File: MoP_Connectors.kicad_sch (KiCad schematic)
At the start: 1 part, among them J22 Conn_02x22_Top_Bottom

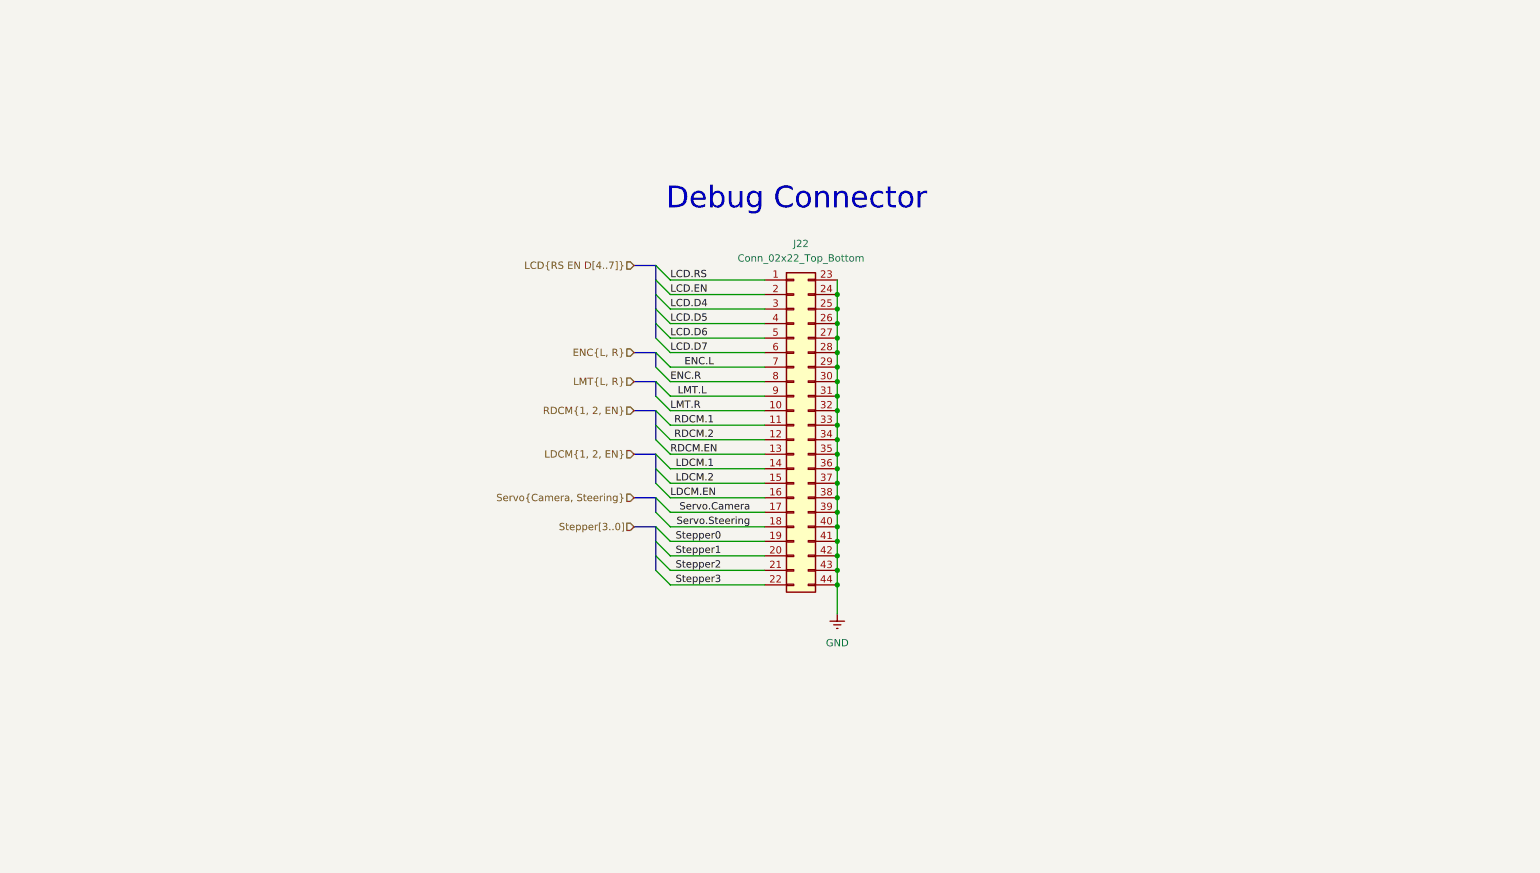
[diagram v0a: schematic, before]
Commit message: Finished schematics
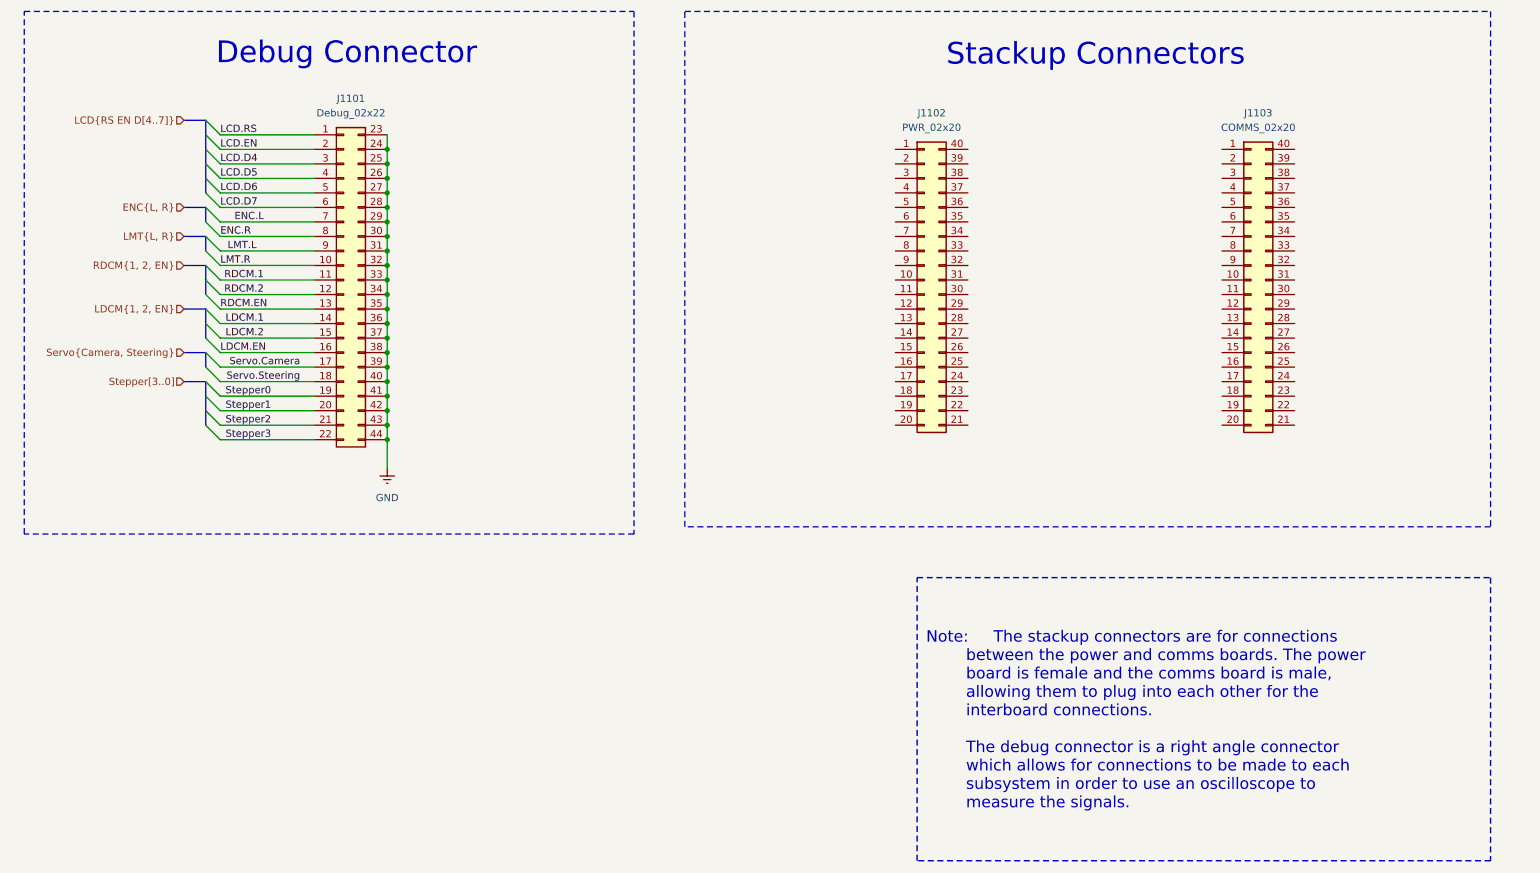
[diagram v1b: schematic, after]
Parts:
- added J1102: PWR_02x20, Connector_PinHeader_2.54mm:PinHeader_2x20_P2.54mm_Vertical, symbol Connector_Generic:Conn_02x20_Counter_Clockwise
- added J1103: COMMS_02x20, Connector_PinHeader_2.54mm:PinHeader_2x20_P2.54mm_Vertical, symbol Connector_Generic:Conn_02x20_Counter_Clockwise
- J1101: renamed from J22; value Conn_02x22_Top_Bottom -> Debug_02x22; footprint (none) -> Connector_PinHeader_1.00mm:PinHeader_2x19_P1.00mm_Vertical
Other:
- note added: "Stackup Connectors"
- moved on the sheet: J1101
